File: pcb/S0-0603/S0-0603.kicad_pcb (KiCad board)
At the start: 2 copper layers, 100 x 40 mm, 9 parts

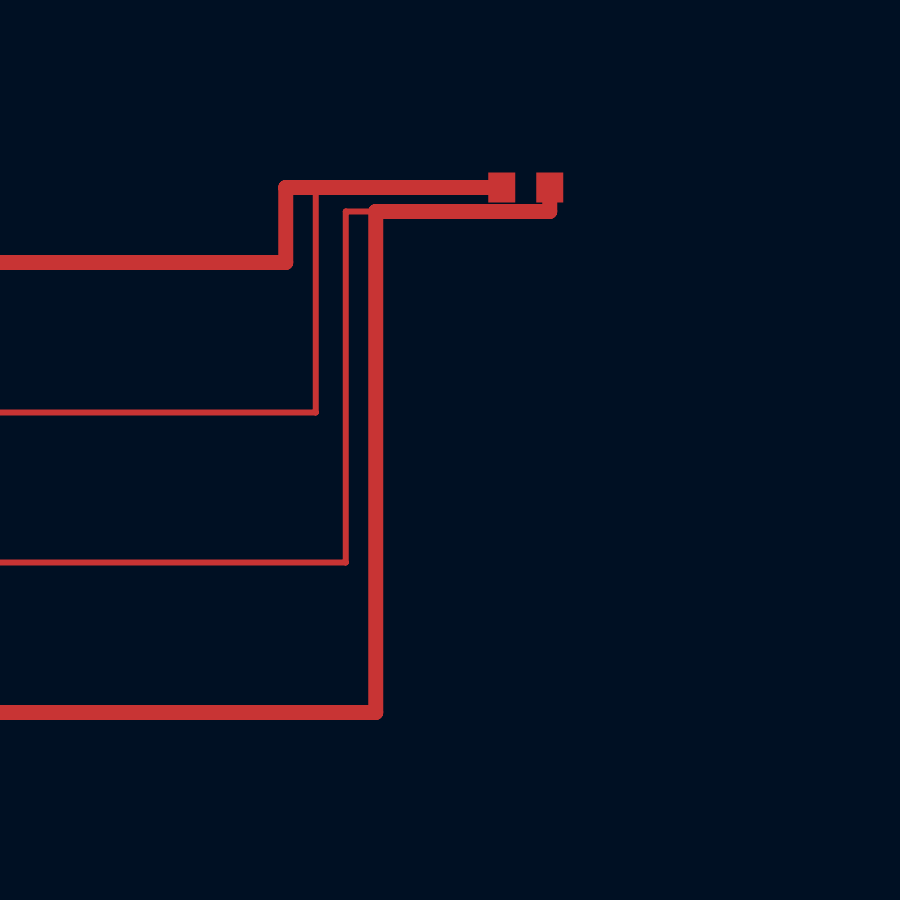
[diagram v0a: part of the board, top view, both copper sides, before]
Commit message: v0.3.1 — PCB CAD & JLCPCB Fabrication Package
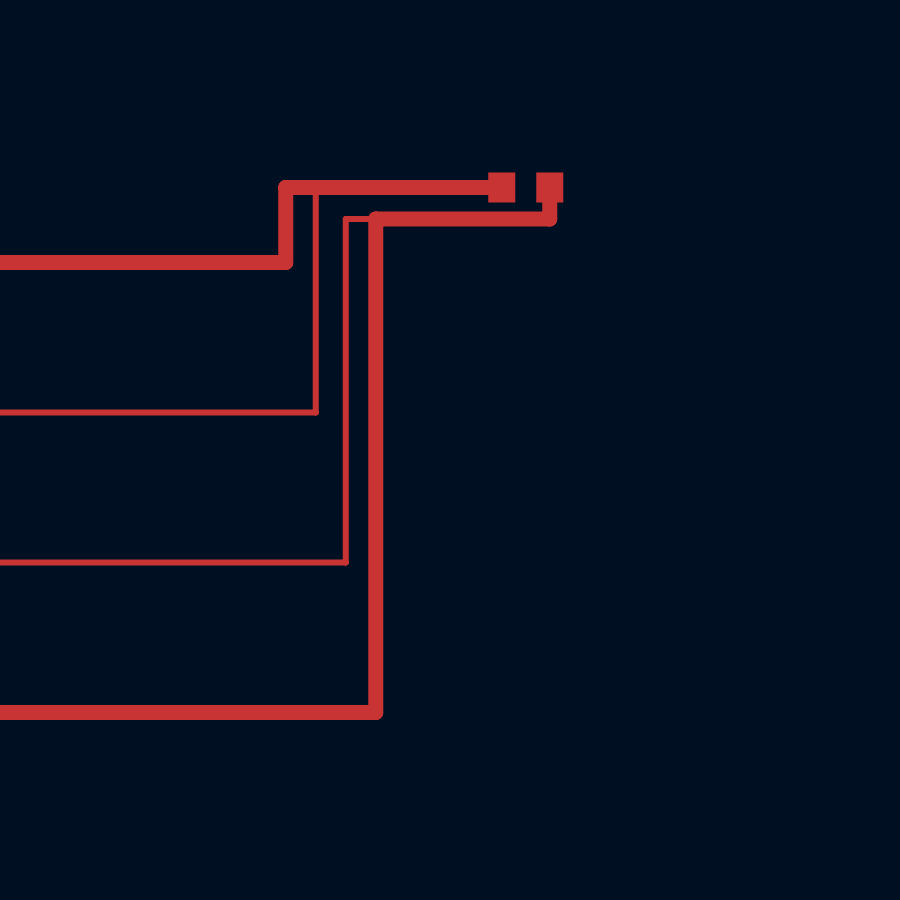
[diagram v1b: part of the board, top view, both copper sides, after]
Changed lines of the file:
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@@
 		(pad "1" smd rect (at -0.8 0) (size 0.9 1.0) (layers "F.Cu" "F.Paste" "F.Mask") (net 1 "DRIVE_SENSE_PLUS"))
 		(pad "2" smd rect (at 0.8 0) (size 0.9 1.0) (layers "F.Cu" "F.Paste" "F.Mask") (net 2 "DRIVE_SENSE_MINUS"))
+		(model "/Applications/KiCad/KiCad.app/Contents/SharedSupport/3dmodels/Capacitor_SMD.3dshapes/C_0603_1608Metric.step"
+			(offset (xyz 0 0 0))
+			(scale (xyz 1 1 1))
+			(rotate (xyz 0 0 0))
+		)
 	)
 	(footprint "SC4:EdgeContact_2.5mm_Round" (layer "F.Cu")
@@
 	(segment (start 43.0 10.0) (end 49.2 10.0) (width 0.2) (layer "F.Cu") (net 1))
 	(segment (start 5.0 22.5) (end 44.0 22.5) (width 0.2) (layer "F.Cu") (net 2))
-	(segment (start 44.0 22.5) (end 44.0 10.8) (width 0.2) (layer "F.Cu") (net 2))
-	(segment (start 44.0 10.8) (end 50.8 10.8) (width 0.2) (layer "F.Cu") (net 2))
-	(segment (start 50.8 10.8) (end 50.8 10.0) (width 0.2) (layer "F.Cu") (net 2))
+	(segment (start 44.0 22.5) (end 44.0 11.05) (width 0.2) (layer "F.Cu") (net 2))
+	(segment (start 44.0 11.05) (end 50.8 11.05) (width 0.2) (layer "F.Cu") (net 2))
+	(segment (start 50.8 11.05) (end 50.8 10.0) (width 0.2) (layer "F.Cu") (net 2))
 	(segment (start 5.0 27.5) (end 45.0 27.5) (width 0.5) (layer "F.Cu") (net 2))
-	(segment (start 45.0 27.5) (end 45.0 10.8) (width 0.5) (layer "F.Cu") (net 2))
-	(segment (start 45.0 10.8) (end 50.8 10.8) (width 0.5) (layer "F.Cu") (net 2))
-	(segment (start 50.8 10.8) (end 50.8 10.0) (width 0.5) (layer "F.Cu") (net 2))
+	(segment (start 45.0 27.5) (end 45.0 11.05) (width 0.5) (layer "F.Cu") (net 2))
+	(segment (start 45.0 11.05) (end 50.8 11.05) (width 0.5) (layer "F.Cu") (net 2))
+	(segment (start 50.8 11.05) (end 50.8 10.0) (width 0.5) (layer "F.Cu") (net 2))
 	(gr_text "S0-0603" (at 5.0 31.0 0) (layer "F.SilkS")
 		(effects (font (size 1 1) (thickness 0.15)))
